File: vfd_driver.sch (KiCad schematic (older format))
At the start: 34 parts, among them J1 Input, J2 futaba_7_lt_44z, J3 High Volt, J4 FIL_n, J5 FIL_p, Q3 BC817, Q4 BC807, Q5 BC817, Q6 BC807, U1 74HC595, U2 74HC595, U3 74HC595, U4 74HC595, U5 TBD62783A, U6 TBD62783A, U7 TBD62783A

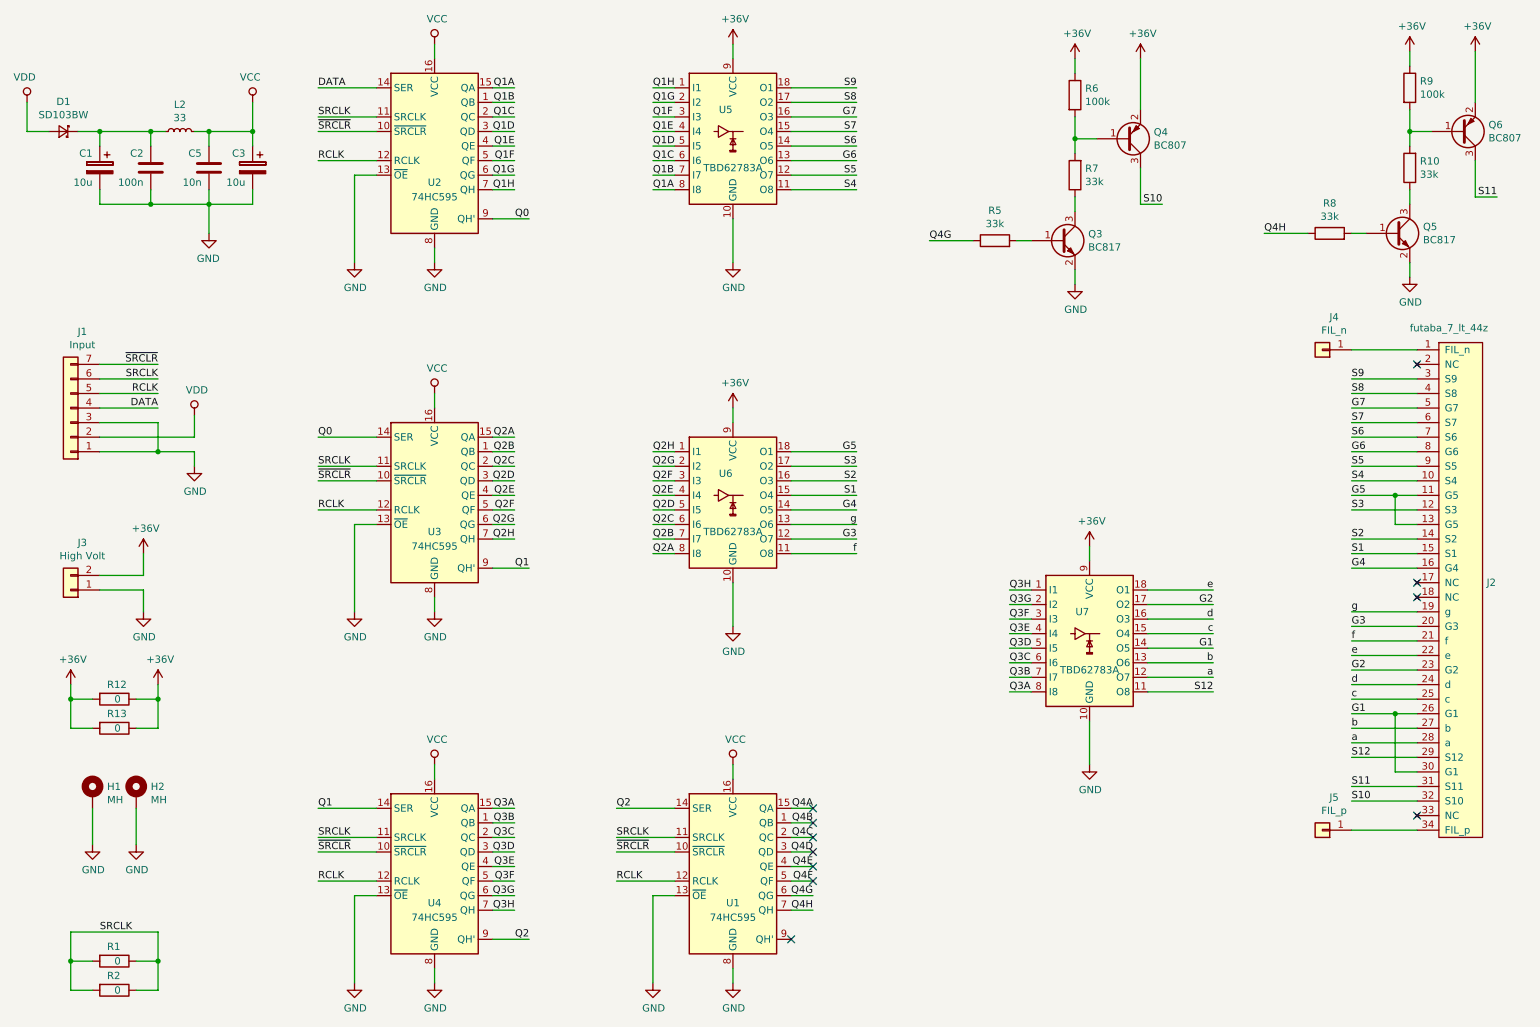
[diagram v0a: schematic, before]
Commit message: before adding lt1073
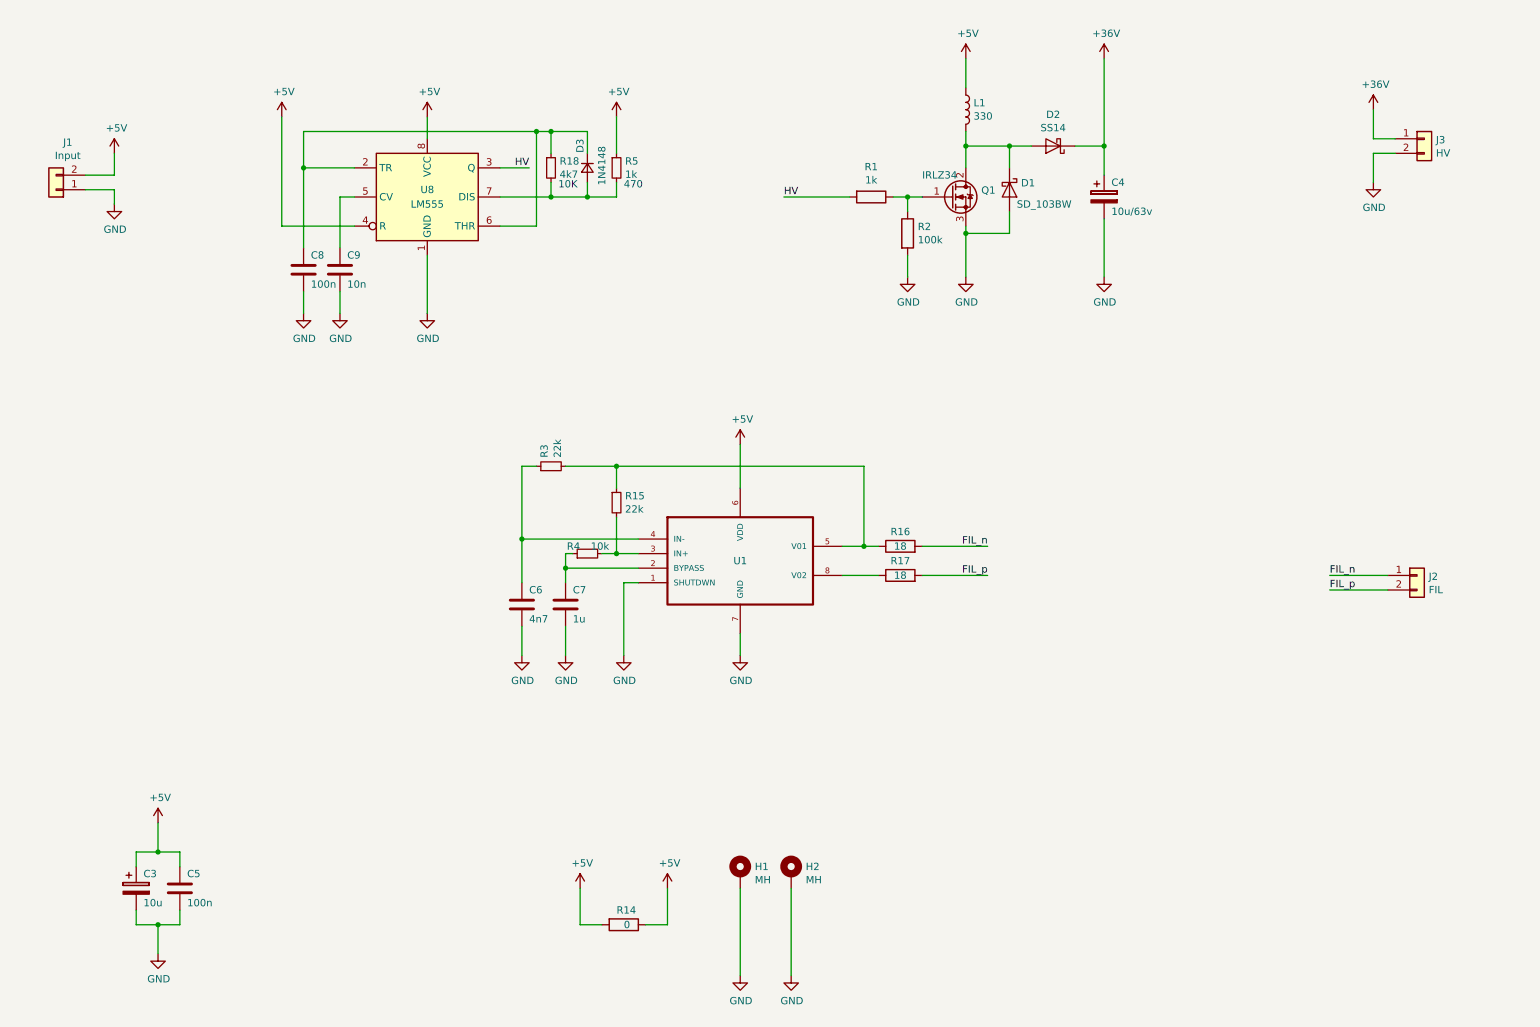
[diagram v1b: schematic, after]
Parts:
- removed C1: 10u, Capacitor_THT:CP_Radial_D8.0mm_P3.80mm, symbol Device:CP
- removed C2: 100n, Capacitor_SMD:C_0805_2012Metric_Pad1.15x1.40mm_HandSolder, symbol Device:C
- removed D1: SD103BW, Diode_SMD:D_SOD-123, symbol Device:D_Schottky_Small
- removed J1: Input, Connector_PinSocket_2.54mm:PinSocket_1x07_P2.54mm_Vertical, symbol Connector_Generic:Conn_01x07
- removed J2: futaba_7_lt_44z, Connector_PinSocket_2.54mm:PinSocket_1x34_P2.54mm_Vertical, symbol vfd_driver-rescue:futaba_7_lt_44z-custom-vfd_driver-rescue
- removed J4: FIL_n, Connector_Pin:Pin_D1.4mm_L8.5mm_W2.8mm_FlatFork, symbol Connector_Generic:Conn_01x01
- removed J5: FIL_p, Connector_Pin:Pin_D1.4mm_L8.5mm_W2.8mm_FlatFork, symbol Connector_Generic:Conn_01x01
- removed L2: 33, Inductor_SMD:L_1206_3216Metric_Pad1.42x1.75mm_HandSolder, symbol Device:L_Small
- removed Q3, Q5: BC817, Package_TO_SOT_SMD:SOT-23, symbol Transistor_BJT:BC817
- removed Q4, Q6: BC807, Package_TO_SOT_SMD:SOT-23, symbol Transistor_BJT:BC807
- removed R10, R5, R7, R8: 33k, Resistor_SMD:R_0805_2012Metric_Pad1.15x1.40mm_HandSolder, symbol Device:R
- removed R12, R13: 0, Resistor_SMD:R_1206_3216Metric, symbol Device:R
- removed R6, R9: 100k, Resistor_SMD:R_0805_2012Metric_Pad1.15x1.40mm_HandSolder, symbol Device:R
- removed U1, U2, U3, U4: 74HC595, Package_SO:SOIC-16_3.9x9.9mm_P1.27mm, symbol 74xx:74HC595
- removed U5, U6, U7: TBD62783A, Package_SO:SOP-18_7.0x12.5mm_P1.27mm, symbol Transistor_Array:TBD62783A
- added C4: 10u/63v, Capacitor_THT:CP_Radial_D8.0mm_P5.00mm, symbol Device:CP
- added C6: 4n7, Capacitor_SMD:C_0805_2012Metric_Pad1.15x1.40mm_HandSolder, symbol Device:C
- added C7: 1u, Capacitor_THT:C_Rect_L7.0mm_W2.0mm_P5.00mm, symbol Device:C
- added C8: 100n, Capacitor_THT:C_Rect_L7.0mm_W2.0mm_P5.00mm, symbol Device:C
- added C9: 10n, Capacitor_SMD:C_0805_2012Metric_Pad1.15x1.40mm_HandSolder, symbol Device:C
- added D1: SD_103BW, Diode_SMD:D_SOD-123, symbol Device:D_Schottky
- added D2: SS14, Diode_SMD:D_SMA_Handsoldering, symbol Device:D_Schottky
- added D3: 1N4148, Diode_SMD:D_MiniMELF, symbol Device:D_Small
- added J1: Input, Connector_PinHeader_2.54mm:PinHeader_1x02_P2.54mm_Vertical, symbol Connector_Generic:Conn_01x02
- added J2: FIL, Connector_PinHeader_2.54mm:PinHeader_1x02_P2.54mm_Vertical, symbol Connector_Generic:Conn_01x02
- added L1: 330, Choke_SMD:Choke_CD75, symbol Device:L
- added Q1: IRLZ34, Package_TO_SOT_THT:TO-220-3_Vertical, symbol Device:Q_NMOS_GDS
- added R14: 0, Resistor_SMD:R_1206_3216Metric, symbol Device:R
- added R15, R3: 22k, Resistor_SMD:R_0805_2012Metric_Pad1.15x1.40mm_HandSolder, symbol Device:R_Small
- added R16, R17: 18, Resistor_SMD:R_1206_3216Metric_Pad1.42x1.75mm_HandSolder, symbol Device:R
- added R18: 4k7, Resistor_SMD:R_0805_2012Metric_Pad1.15x1.40mm_HandSolder, symbol Device:R_Small
- added R4: 10k, Resistor_SMD:R_0805_2012Metric_Pad1.15x1.40mm_HandSolder, symbol Device:R_Small
- added R5: 1k, Resistor_SMD:R_0805_2012Metric_Pad1.15x1.40mm_HandSolder, symbol Device:R_Small
- added U1: LM4871, Package_SO:SOIC-8_3.9x4.9mm_P1.27mm, symbol vfd_driver-rescue:LM4871-LM4871
- added U8: LM555, Package_DIP:DIP-8_W7.62mm_Socket_LongPads, symbol Timer:LM555
- C5: value 10n -> 100n
- J3: value High Volt -> HV
- R1: value 0 -> 1k; footprint Resistor_SMD:R_1206_3216Metric -> Resistor_SMD:R_0805_2012Metric_Pad1.15x1.40mm_HandSolder
- R2: value 0 -> 100k; footprint Resistor_SMD:R_1206_3216Metric -> Resistor_SMD:R_0805_2012Metric_Pad1.15x1.40mm_HandSolder
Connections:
- net +36V: now also J3.1 (Pin_1), C4.1, D2.1 (K); no longer J3.2 (Pin_2)
- net GND: now also J3.2 (Pin_2), R2.2, C4.2, C6.2, C7.2, C8.2, C9.2, D1.2 (A), J1.1 (Pin_1), Q1.3 (S), U1.1 (SHUTDWN), U1.7 (GND), U8.1 (GND); no longer J3.1 (Pin_1)
- net SRCLK: no longer names the net of R1.1, R2.1
- net SRCLK: now also Q1.1 (G); no longer R1.2, R2.2
- net VCC renamed +5V
- net +5V: now also J1.2 (Pin_2), L1.1, R14.1, R14.2, R5.1, U1.6 (VDD), U8.4 (R), U8.8 (VCC)
- new net: D1.1 (K), D2.2 (A), L1.2, Q1.2 (D)
- new net: D3.2 (A), R18.2, R5.2, U8.7 (DIS)
- new net: C8.1, D3.1 (K), R18.1, U8.2 (TR), U8.6 (THR)
- new net: C9.1, U8.5 (CV)
- new net: C7.1, R4.1, U1.2 (BYPASS)
- new net: R15.2, R4.2, U1.3 (IN+)
- new net: C6.1, R3.1, U1.4 (IN-)
- new net: R15.1, R16.1, R3.2, U1.5 (V01)
- new net: R17.1, U1.8 (V02)
- new net FIL_n: J2.1 (Pin_1), R16.2
- new net FIL_p: J2.2 (Pin_2), R17.2
- new net HV: R1.2, U8.3 (Q)
- no-connect marks 11 -> 0
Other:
- note added: "10K"
- note added: "470"
- moved on the sheet: C3, C5, H1, H2
